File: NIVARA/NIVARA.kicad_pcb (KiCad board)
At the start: 2 copper layers, 69 parts, among them J10 PNP INPUT, J11 Screw_Terminal_01x02, J12 PNP OUTPUT, J13 Salidas AN, J16 Salida An 4-20mA, J3 Entrada An 0-10V, J4 Entrada An 0-32V, J5 Relay, J6 Entrada An 5-20mA, J7 NPN INPUT, J8 RS485, J9 NPN OUTPUT, K1 SANYOU_SRD_Form_C, K2 SANYOU_SRD_Form_C, Q1 NCV8402xST, Q2 NCV8402xST, Q3 NCV8402xST, Q4 NCV8402xST, U1 ESP32-S3-WROOM-1, U10 LTV-357T, U11 LTV-357T, U13 LTV-357T, U14 LTV-357T, U3 AP63200WU, U4 LTV-357T, U5 LTV-357T, U6 LTV-357T, U7 LTV-357T, U8 LTV-357T, U9 LTV-357T

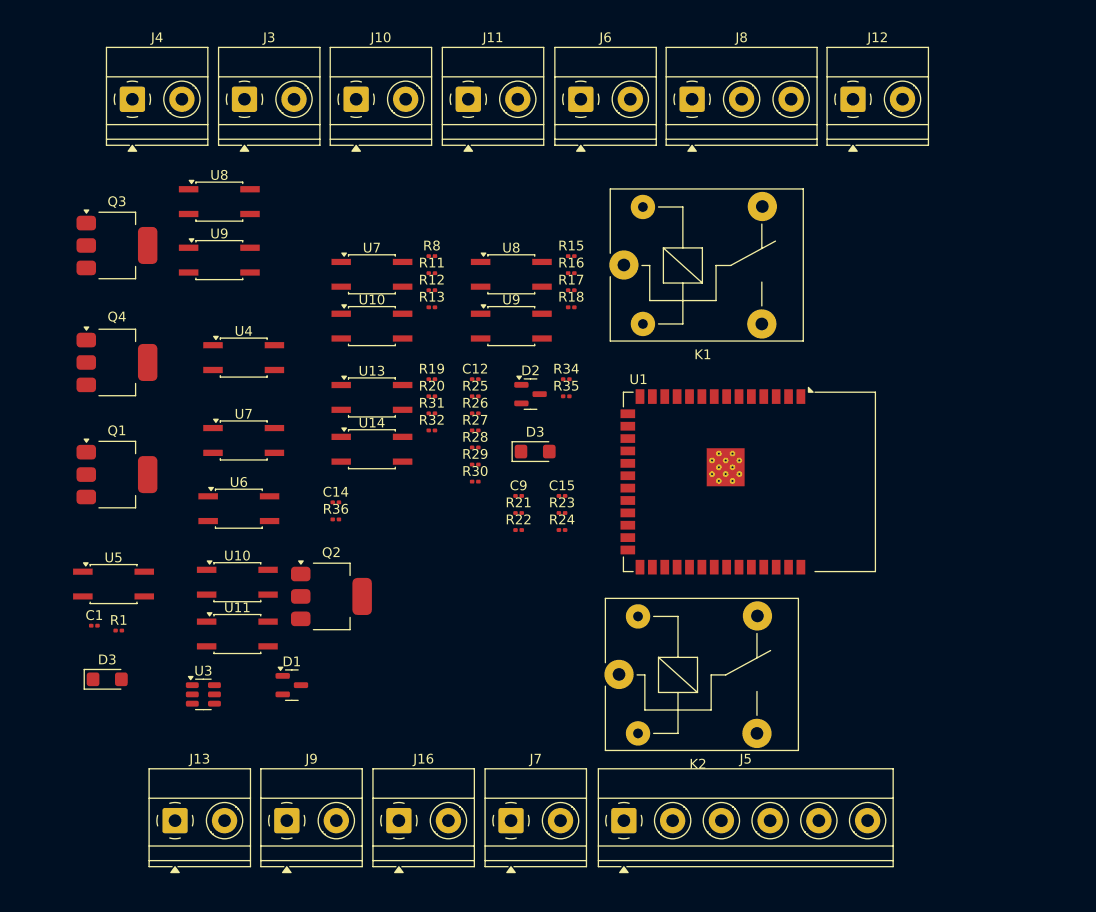
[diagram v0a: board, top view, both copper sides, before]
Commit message: arreglo
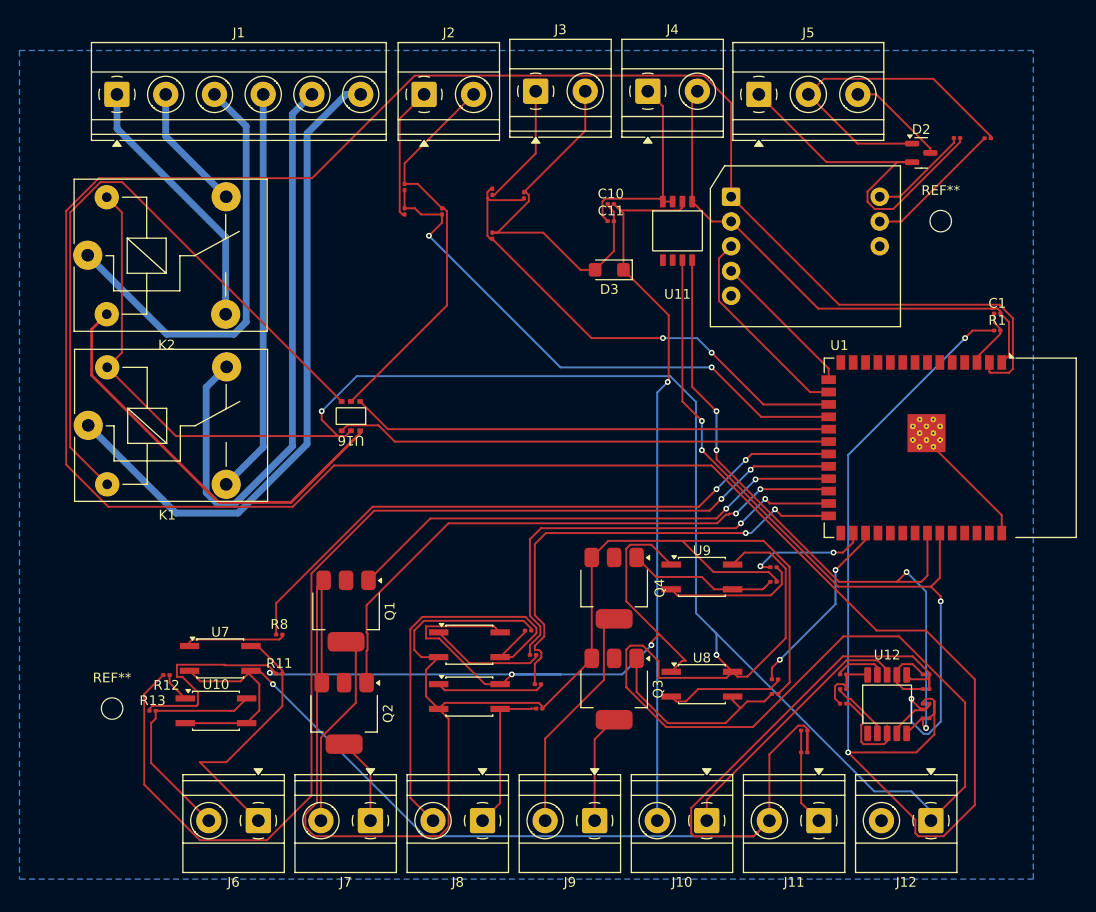
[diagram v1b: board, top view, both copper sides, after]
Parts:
- removed D1: SM712_SOT23, Package_TO_SOT_SMD:SOT-23
- removed the D3 at (58.5, 112.5)
- removed the U10 at (71.8, 102.5)
- removed U3: AP63200WU, Package_TO_SOT_SMD:TSOT-23-6
- removed U4, U5, U6: LTV-357T, Package_SO:SO-4_4.4x3.6mm_P2.54mm
- removed the U7 at (72.5, 88.0)
- removed the U8 at (70.0, 63.5)
- removed the U9 at (70.0, 69.5)
- added C10: 100nF, Capacitor_SMD:C_0201_0603Metric, F.Cu at (110.2, 63.8)
- added C11: 1uF, Capacitor_SMD:C_0201_0603Metric, F.Cu at (110.2, 65.5)
- added REF**: MountingHole_2.2mm_M2, MountingHole:MountingHole_2.2mm_M2, F.Cu at (59.0, 115.5)
- added REF**: MountingHole_2.2mm_M2, MountingHole:MountingHole_2.2mm_M2, F.Cu at (144.0, 65.5)
- added U12: ~, Project Library:GP8303, F.Cu at (138.5, 115.0)
- added U15: ~, Project Library:RSM3485ECHT, F.Cu at (129.9, 69.3)
- added U16: ~, Project Library:LK1802, F.Cu at (83.5, 85.5)
- U11: value LTV-357T -> ~; footprint Package_SO:SO-4_4.4x3.6mm_P2.54mm -> Project Library:GP8201S
- moved C1 98.0 mm to (149.8, 75.0)
- moved R1 95.2 mm to (149.8, 76.7)
- moved J1 90.9 mm to (59.5, 52.5)
- moved J12 87.9 mm to (143.0, 127.0), turned to 180 degrees
- moved J9 78.6 mm to (108.5, 127.0), turned to 180 degrees
- moved J8 75.1 mm to (97.0, 127.0), turned to 180 degrees
- moved K2 69.4 mm to (56.5, 69.0)
- moved Q3 68.3 mm to (110.5, 113.5), turned to -90 degrees
- moved U11 61.2 mm to (117.0, 66.5)
- moved K1 57.4 mm to (56.5, 86.5)
- moved Q4 56.0 mm to (110.5, 103.2), turned to -90 degrees
- moved R25 56.0 mm to (142.5, 115.0)
- moved C12 55.3 mm to (142.5, 112.0)
- moved R27 54.9 mm to (142.5, 116.5)
- moved J10 54.5 mm to (120.0, 127.0), turned to 180 degrees
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- renumbered J5 to J1, J13 to J10, J16 to J11, J11 to J12, J3 to J2, J4 to J3, J6 to J4, J8 to J5, J7 to J6, J9 to J7, J10 to J8, J12 to J9
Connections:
- J1 pad 5: /NIVARA/RLY1_NC -> /NIVARA/RLY1_C
- J7 pad 1: /NIVARA/NPN_OUT_1 -> /NIVARA/NPN_OUT_2
- J7 pad 2: /NIVARA/NPN_OUT_2 -> /NIVARA/NPN_OUT_1
- J8 pad 1: /NIVARA/PNP_IN_1 -> /NIVARA/PNP_IN_2
- J8 pad 2: /NIVARA/PNP_IN_2 -> /NIVARA/PNP_IN_1
- K1 pad 4: /NIVARA/RLY1_NC -> /NIVARA/RLY1_C
- U1 pad 1: Net-(U1-GND-Pad1) -> GND
- U1 pad 12: /NIVARA/PNP_OUT/PNP_OUT_IN_1 -> unconnected-(U1-GPIO8/TOUCH8/ADC1_CH7/SUBSPICS1-Pad12)
- U1 pad 15: /NIVARA/RELE_IN/RELAY2_IN -> /NIVARA/RS485_drivers/RS485_IN
- U1 pad 16: unconnected-(U1-GPIO46-Pad16) -> /NIVARA/RS485_drivers/RS485_OUT
- U1 pad 17: /NIVARA/PNP_OUT/PNP_OUT_IN_2 -> /NIVARA/A_IN_32V/32V_A_IN_OUT
- U1 pad 18: /NIVARA/PNP_IN/PNP_IN_IN_1 -> /NIVARA/A_IN_10V/10V_A_IN_OUT
- U1 pad 19: /NIVARA/PNP_IN/PNP_IN_IN_2 -> /NIVARA/RELE_IN/RELAY1_IN
- U1 pad 2: unconnected-(U1-3V3-Pad2) -> +3.3V
- U1 pad 20: /NIVARA/A_IN_10V/10V_A_IN_OUT -> /NIVARA/RELE_IN/RELAY2_IN
- U1 pad 21: /NIVARA/A_IN_32V/32V_A_IN_OUT -> /NIVARA/NPN_IN/NPN_IN_IN_1
- U1 pad 22: unconnected-(U1-GPIO14/TOUCH14/ADC2_CH3/FSPIWP/FSPIDQS/SUBSPIWP-Pad22) -> /NIVARA/NPN_IN/NPN_IN_IN_2
- U1 pad 23: unconnected-(U1-GPIO21-Pad23) -> /NIVARA/NPN_OUT/NPN_OUT_IN_1
- U1 pad 24: unconnected-(U1-GPIO47/SPICLK_P/SUBSPICLK_P_DIFF-Pad24) -> /NIVARA/NPN_OUT/NPN_OUT_IN_2
- U1 pad 25: unconnected-(U1-GPIO48/SPICLK_N/SUBSPICLK_N_DIFF-Pad25) -> /NIVARA/PNP_IN/PNP_IN_IN_1
- U1 pad 26: unconnected-(U1-GPIO45-Pad26) -> /NIVARA/PNP_IN/PNP_IN_IN_2
- U1 pad 28: unconnected-(U1-SPIIO6/GPIO35/FSPID/SUBSPID-Pad28) -> /NIVARA/PNP_OUT/PNP_OUT_IN_2
- U1 pad 29: unconnected-(U1-SPIIO7/GPIO36/FSPICLK/SUBSPICLK-Pad29) -> /NIVARA/PNP_OUT/PNP_OUT_IN_1
- U1 pad 36: /NIVARA/RS485_drivers/RS485_IN -> unconnected-(U1-U0RXD/GPIO44/CLK_OUT2-Pad36)
- U1 pad 37: /NIVARA/RS485_drivers/RS485_OUT -> unconnected-(U1-U0TXD/GPIO43/CLK_OUT1-Pad37)
- U1 pad 38: /NIVARA/RELE_IN/RELAY1_IN -> unconnected-(U1-GPIO2/TOUCH2/ADC1_CH1-Pad38)
- U1 pad 39: /NIVARA/A_OUT_420mA -> unconnected-(U1-GPIO1/TOUCH1/ADC1_CH0-Pad39)
- U1 pad 4: /NIVARA/NPN_OUT/NPN_OUT_IN_1 -> unconnected-(U1-GPIO4/TOUCH4/ADC1_CH3-Pad4)
- U1 pad 40: Net-(U1-GND-Pad1) -> GND
- U1 pad 41: Net-(U1-GND-Pad1) -> GND
- U1 pad 5: /NIVARA/NPN_OUT/NPN_OUT_IN_2 -> unconnected-(U1-GPIO5/TOUCH5/ADC1_CH4-Pad5)
- U1 pad 6: /NIVARA/NPN_IN/NPN_IN_IN_1 -> unconnected-(U1-GPIO6/TOUCH6/ADC1_CH5-Pad6)
- U1 pad 7: /NIVARA/NPN_IN/NPN_IN_IN_2 -> unconnected-(U1-GPIO7/TOUCH7/ADC1_CH6-Pad7)
- U10 pad 2: GNDPWR -> GND
- U11 pad 1: Net-(R25-Pad2) -> /NIVARA/V_ANAG_OUT/SCLK
- U11 pad 2: unconnected-(U11-Pad2) -> /NIVARA/V_ANAG_OUT/SDA
- U11 pad 3: Net-(Q2-G) -> unconnected-(U11-NC-Pad3)
- U11 pad 4: +3.3V -> VCC
- U13 pad 2: GNDPWR -> GND
- U14 pad 2: GNDPWR -> GND
- U7 pad 2: GNDPWR -> GND
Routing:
- net +3.3V: track 0.00 -> 469.1 mm, vias 0 -> 5
- net GND: track 0.00 -> 467.7 mm, vias 0 -> 1
- net VCC: track 0.00 -> 247.5 mm, vias 0 -> 2
- net /NIVARA/RLY1_C: track 0.00 -> 130.7 mm
- net /NIVARA/NPN_IN/NPN_IN_IN_2: track 0.00 -> 113.8 mm, vias 0 -> 2
- net /NIVARA/V_ANAG_OUT/SDA: track 0.00 -> 83.6 mm, vias 0 -> 4
- net /NIVARA/V_ANAG_OUT/SCLK: track 0.00 -> 74.6 mm, vias 0 -> 4
- net /NIVARA/V_AN_OUT: track 0.00 -> 74.1 mm, vias 0 -> 1
- net Net-(U16-1C): track 0.00 -> 67.9 mm
- net /NIVARA/NPN_IN/NPN_IN_IN_1: track 0.00 -> 66.2 mm, vias 0 -> 2
- net /NIVARA/NPN_OUT/NPN_OUT_IN_2: track 0.00 -> 60.4 mm, vias 0 -> 2
- net /NIVARA/A_IN_10V/10V_A_IN_OUT: track 0.00 -> 57.4 mm, vias 0 -> 2
- net /NIVARA/NPN_OUT/NPN_OUT_IN_1: track 0.00 -> 51.5 mm, vias 0 -> 2
- net /NIVARA/A_IN_32V/32V_A_IN_OUT: track 0.00 -> 51.2 mm, vias 0 -> 2
- net /NIVARA/RELE_IN/RELAY2_IN: track 0.00 -> 50.9 mm
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- added copper zone on B.Cu, net GND
